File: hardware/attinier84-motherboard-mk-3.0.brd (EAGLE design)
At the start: 34 x 29 mm, 8 parts, among them IC1 ATTINY84, U1 ATTINIER84_SHIELD1551GSMD

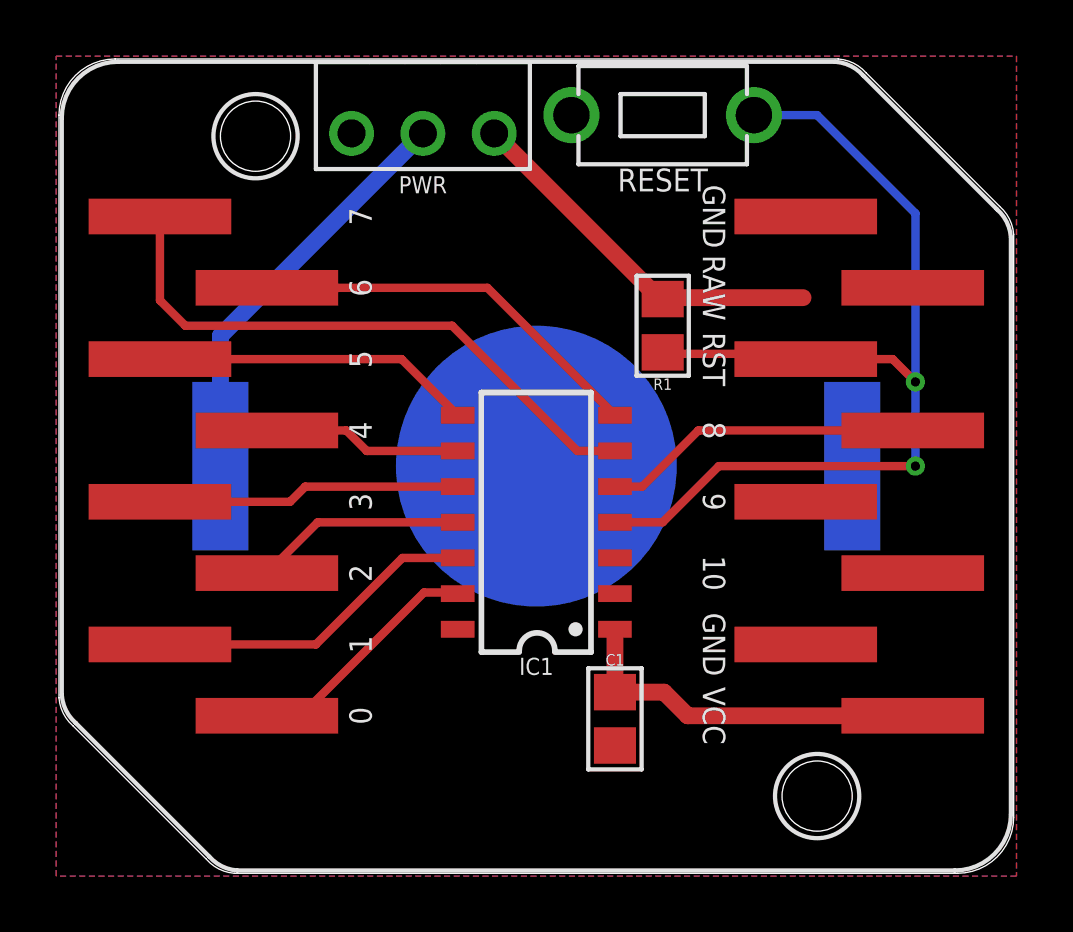
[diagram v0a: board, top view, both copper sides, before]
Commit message: finished up motherboard, initial shield dicking
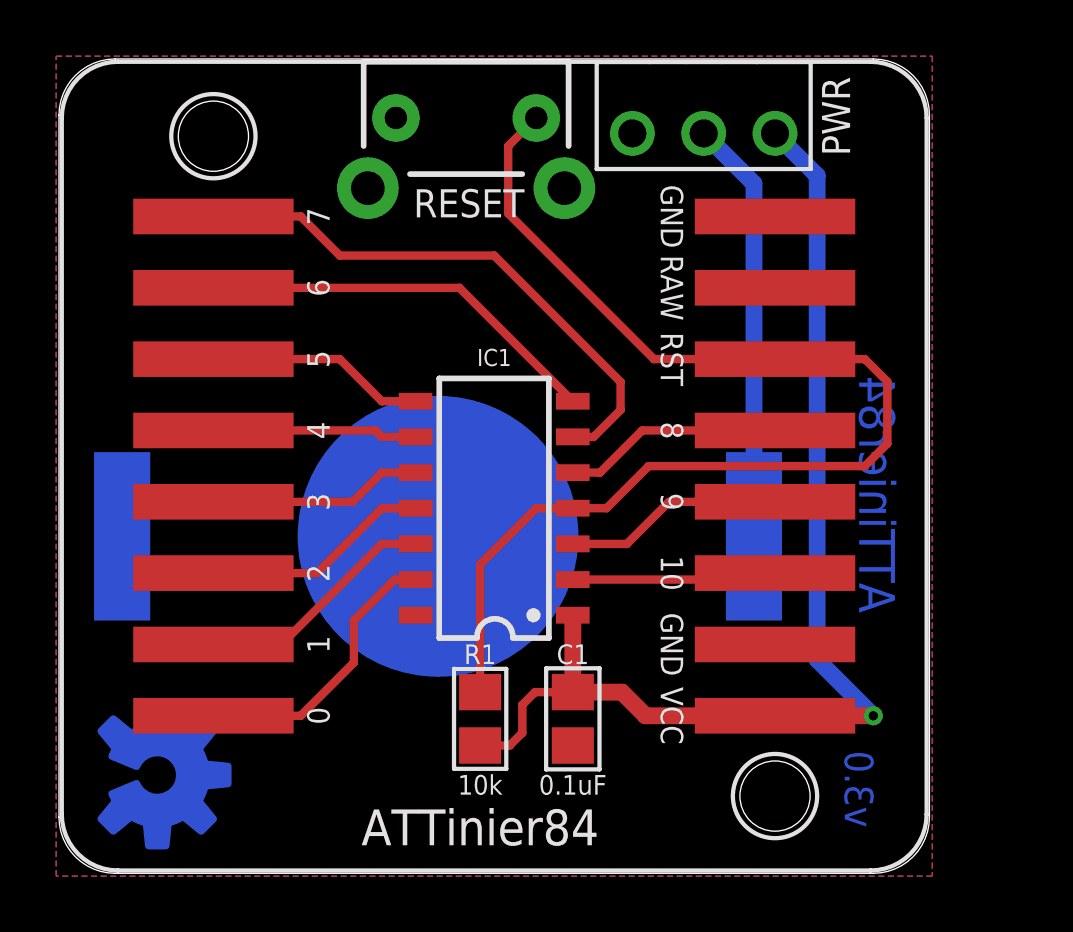
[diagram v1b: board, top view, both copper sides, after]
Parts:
- added U$1: (no value), A_butts:CC-BY-SA-4.0-NO-URL
- added U$2: (no value), A_butts:COW_SMALL
- added U$4: (no value), A_butts:OSHWLOGO_BOT_0.2_A
- RESET: value SPST-NO-TACT3MM-PTH-SMALL-PADS -> SPST-NO-TACT3MM-RA; device A_butts:DTS-3-SMALL-PADS -> A_butts:TACTILE-PTH-SIDE
- moved R1 15.4 mm to (15.0, 5.50), turned to 270 degrees
- moved PWR 10.0 mm to (25.5, 26.4)
- moved RESET 7.00 mm to (14.5, 26.9)
- moved BATT 4.30 mm to (13.5, 12.0)
- moved IC1 1.58 mm to (15.5, 13.0)
- moved C1 1.50 mm to (18.3, 5.50)
- moved U1 1.50 mm to (15.5, 14.5)
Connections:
- net N$1: now also BATT.TOP@2; no longer BATT.TOP@1
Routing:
- net VCC: track 26.7 -> 40.7 mm, vias 0 -> 1
- net PB1: track 0.00 -> 7.82 mm
- net PB0: track 0.00 -> 7.30 mm
- net RST: track 37.2 -> 42.8 mm, vias 2 -> 0
- net PB2: track 11.4 -> 7.82 mm
- net PA5: track 11.4 -> 7.82 mm
- net PA3: track 10.8 -> 7.63 mm
- net PA1: track 11.9 -> 8.68 mm
- net PA0: track 8.63 -> 10.1 mm
- net PA7: track 21.4 -> 20.0 mm
- net PA2: track 7.54 -> 8.16 mm
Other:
- board size 34 x 29 mm -> 31 x 29 mm
- board text added: "+ side up"
- board text added: ">REVISION"
- board text added: "ATTinier84"
